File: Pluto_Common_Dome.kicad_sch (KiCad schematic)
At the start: 47 parts

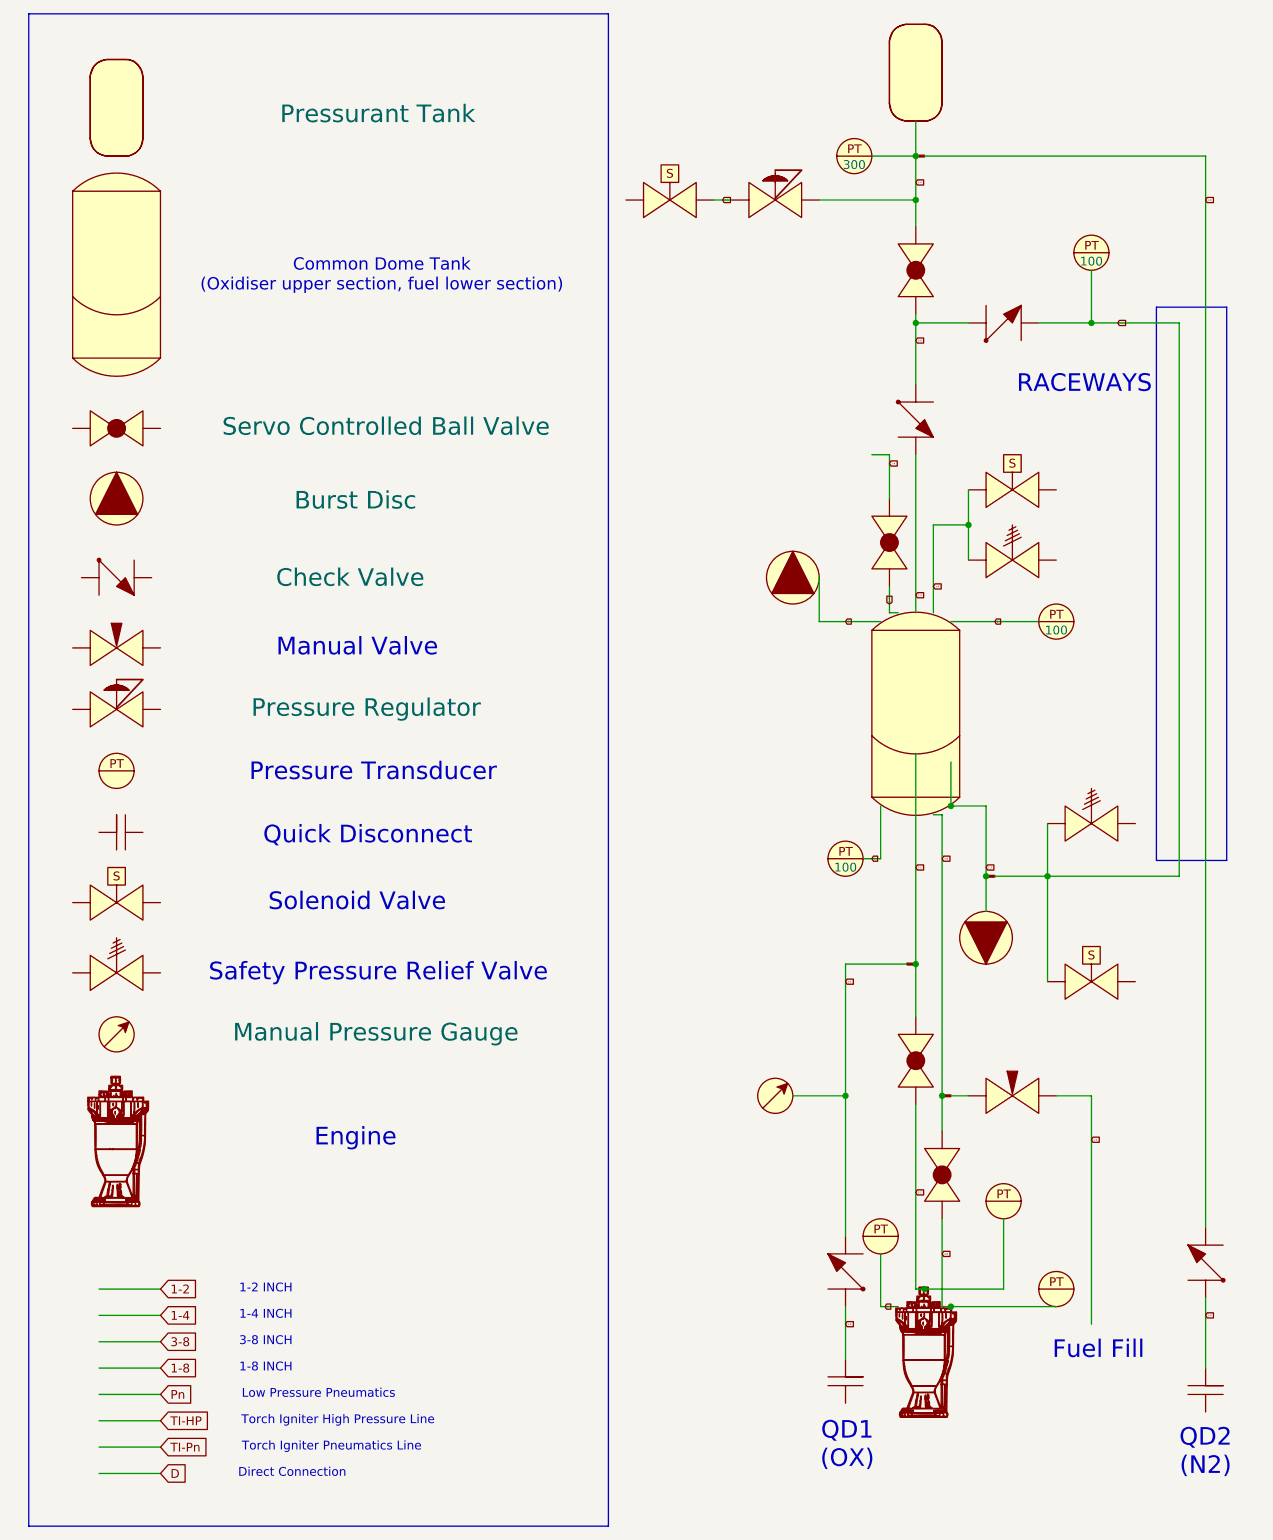
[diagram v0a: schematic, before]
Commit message: more silwood stuff
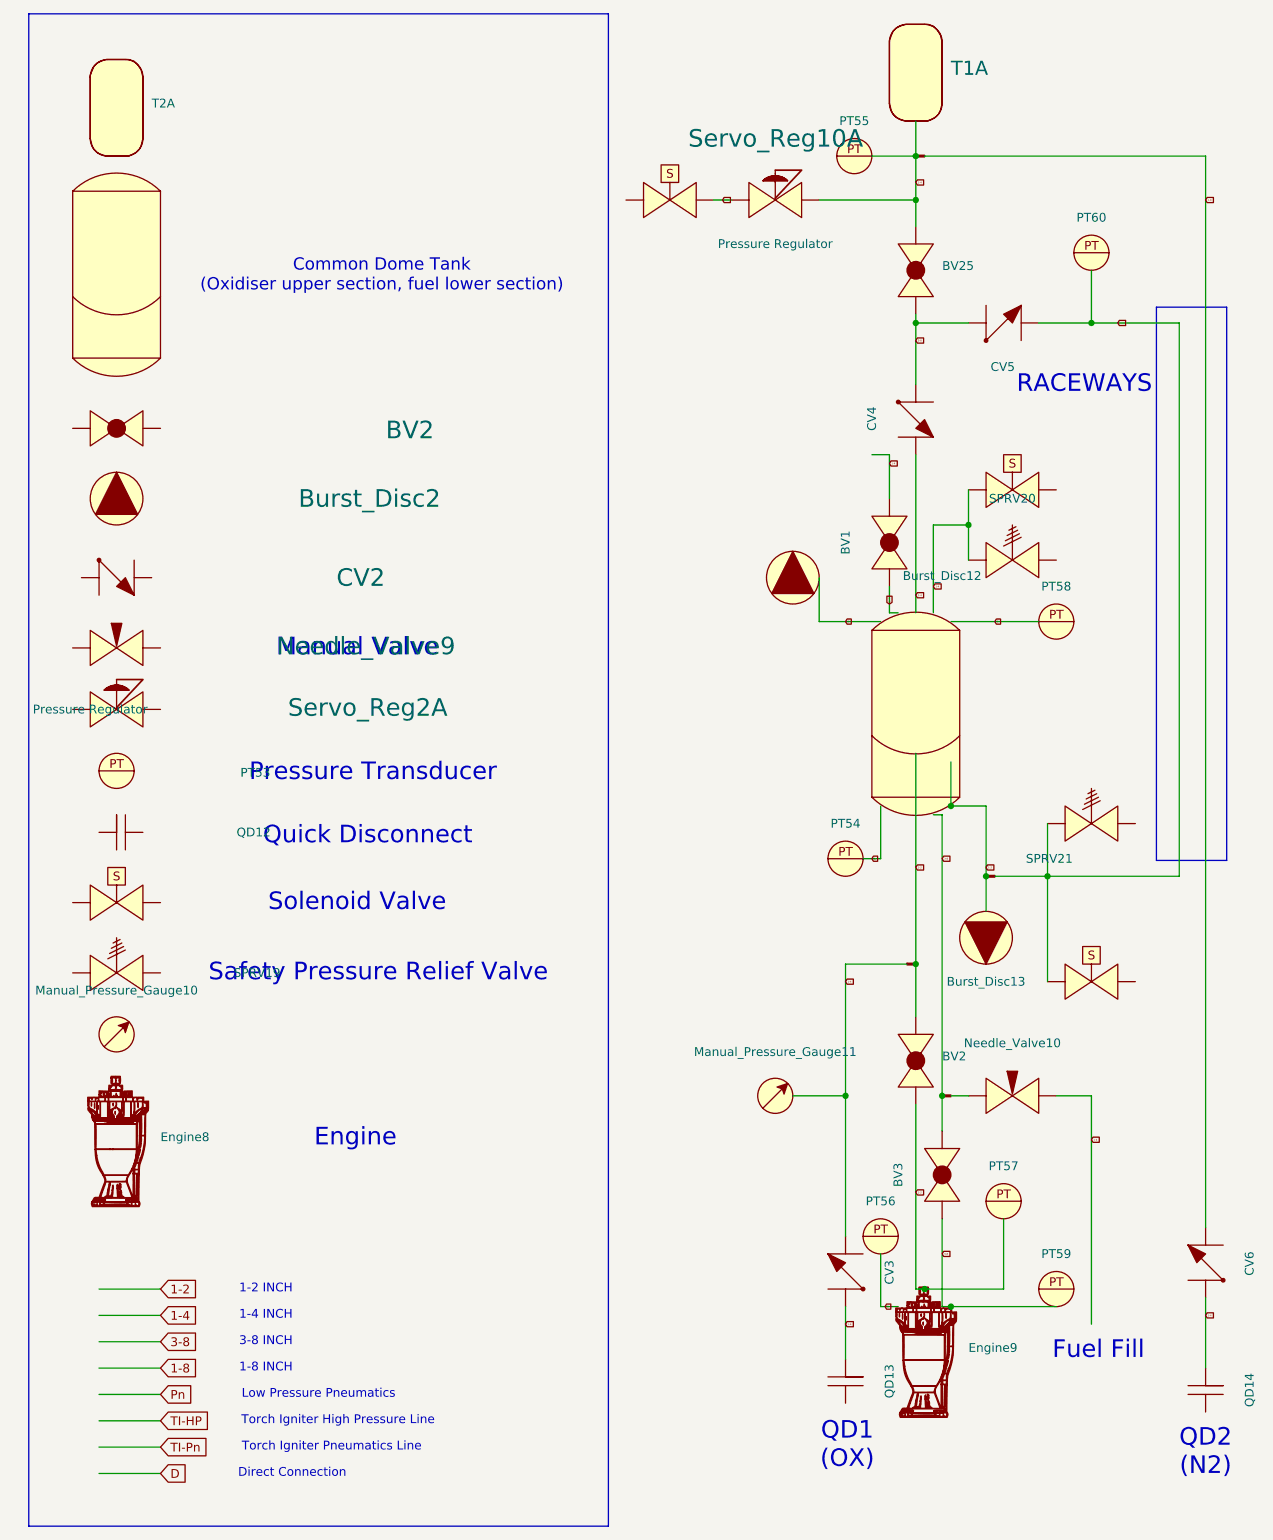
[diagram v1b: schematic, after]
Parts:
- renumbered Ball_Valve1 to BV1, Ball_Valve2 to BV2, Ball_Valve(ServoControlled)2 to BV2, BV26 to BV25, Ball_Valve3 to BV3, BurstDisc2 to Burst_Disc2, Check_Valve4 to CV2, Check_Valve6 to CV3, Check_Valve3 to CV4, Check_Valve2 to CV5, Check_Valve5 to CV6, Engine7 to Engine8, Engine8 to Engine9, Manual_Pressure_Gauge8 to Manual_Pressure_Gauge10, Manual_Pressure_Gauge9 to Manual_Pressure_Gauge11, PT43 to PT53, PT44 to PT54, PT40 to PT55, PT46 to PT56, PT45 to PT57, PT42 to PT58, PT47 to PT59, PT41 to PT60, QD11 to QD12, QD12 to QD13, QD13 to QD14, SPRV17 to SPRV20, SPRV18 to SPRV21, Reg10 to Servo_Reg10, Pressure_Regulator2 to Servo_Reg2, Solenoid7 to Solenoid5, Solenoid5 to Solenoid6, Solenoid6 to Solenoid7, NitrogenTank1 to T1, Tank2 to T2, U38 to U51, U36 to U52, U39 to U53, U37 to U54
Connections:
- new net: Needle_Valve10., U53.

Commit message: Formatiing
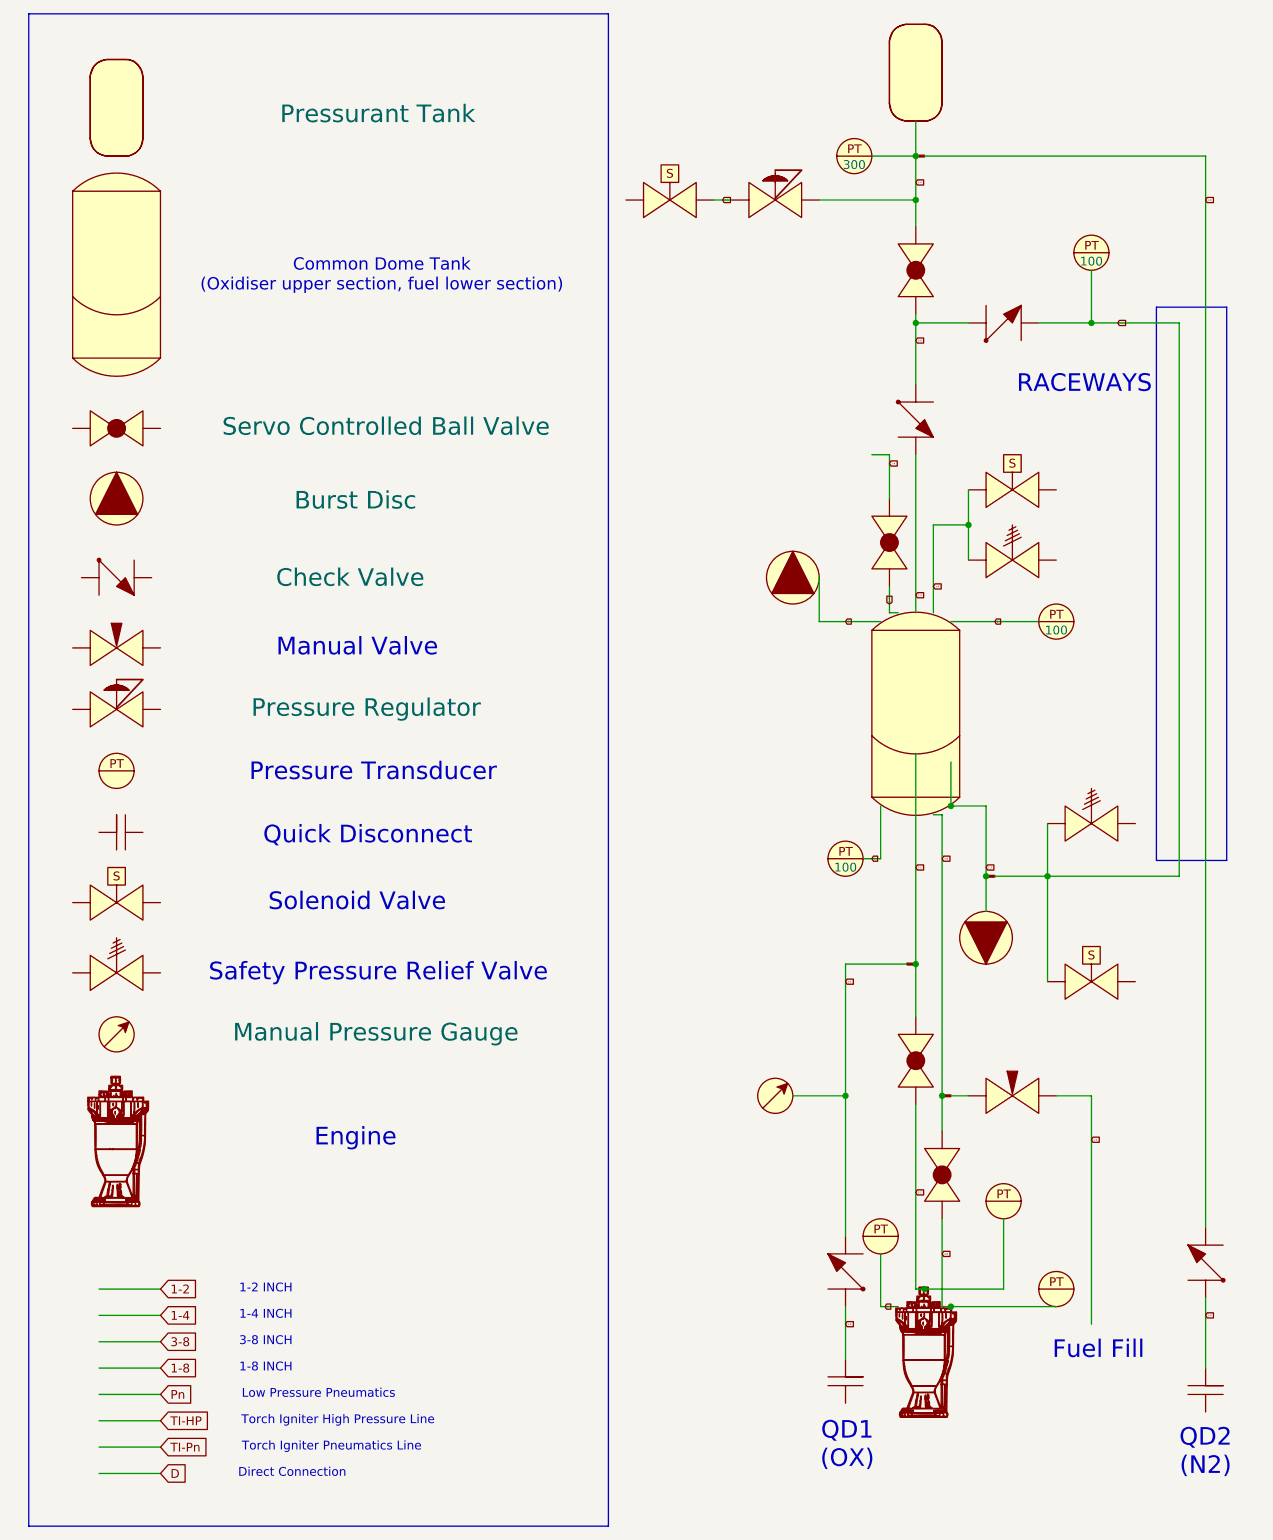
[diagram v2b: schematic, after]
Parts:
- renumbered BV25 to BV52, BV2 to Ball_Valve(ServoControlled)4, BV1 to Ball_Valve7, BV2 to Ball_Valve8, BV3 to Ball_Valve9, Burst_Disc2 to BurstDisc4, Burst_Disc12 to Burst_Disc22, Burst_Disc13 to Burst_Disc23, CV2 to Check_Valve12, CV3 to Check_Valve13, CV4 to Check_Valve14, CV5 to Check_Valve15, CV6 to Check_Valve16, CommonDomeTank1 to CommonDomeTank5, CommonDomeTank2 to CommonDomeTank6, Engine8 to Engine16, Engine9 to Engine17, Manual_Pressure_Gauge11 to Manual_Pressure_Gauge10, Manual_Pressure_Gauge10 to Manual_Pressure_Gauge9, Needle_Valve9 to Needle_Valve15, Needle_Valve10 to Needle_Valve16, T1 to NitrogenTank3, PT53 to PT86, PT54 to PT87, PT55 to PT88, PT56 to PT89, PT57 to PT90, PT58 to PT91, PT59 to PT92, PT60 to PT93, Servo_Reg2 to Pressure_Regulator4, QD12 to QD35, QD13 to QD36, QD14 to QD37, Servo_Reg10 to Reg22, SPRV19 to SPRV29, SPRV20 to SPRV30, SPRV21 to SPRV31, Solenoid5 to Solenoid17, Solenoid6 to Solenoid18, Solenoid7 to Solenoid19, Solenoid8 to Solenoid20, T2 to Tank4, U51 to U49, U52 to U50, U53 to U51, U54 to U52
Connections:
- new net: Needle_Valve16., U51.
